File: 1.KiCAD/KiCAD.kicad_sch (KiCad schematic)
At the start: 22 parts, among them J1 Conn_02x20_Odd_Even, J10 CELL_1, J11 CELL_2, J12 CELL_3, J13 CELL_4, J2 Conn_02x20_Odd_Even, J3 TEMP, J4 TEMP, J5 BAT+, J6 BAT-, J7 LOAD+, J8 LOAD-, Q1 Charge, Q2 Discharge, Q3 Charge, Q4 Discharge, U1 MUX, U2 MUX

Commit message: BOM finished
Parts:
- added C3, C4: 100NF_50V_CER, VAMK_C_SMD:C1206, symbol VAMK_C_SMD:100NF_50V_CER
- added D1, D2: 3.3V, Diode_SMD:D_SMF, symbol Diode:BZV55B3V0
- added R3, R4, R7, R8: 10k, VAMK_R_SMD:1206, symbol VAMK_R_SMD:10k
- added R5: 1m, VAMK_R_SMD:1206, symbol VAMK_R_SMD:0R
- added R6: 160R, VAMK_R_SMD:1206, symbol VAMK_R_SMD:0R
- added U3, U4: AD8021AR, Package_SO:SOIC-8_3.9x4.9mm_P1.27mm, symbol Amplifier_Operational:AD8021AR
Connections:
- net LOAD+ is gone; now on net BAT+: J7.1 (Pin_1)
- net BAT+: now also C1.1, C4.1, R3.2, U3.8 (VS+), U4.4 (+iN), U4.8 (VS+)
- net BAT-: now also C3.2, R5.1, R6.1; no longer C1.1, Q2.1 (S), Q4.1 (S)
- net GND: now also J1.8 (Pin_8), U1.3 (GND), U2.3 (GND), R4.1, R8.1, U4.5 (VS-), U4.6 (REF)
- net PA0: now also J1.28 (Pin_28), J3.2 (Pin_2), R1.2; no longer J1.36 (Pin_36), Q2.4 (G), Q4.4 (G)
- net PA1: now also J1.30 (Pin_30), J4.2 (Pin_2), R2.2; no longer J1.34 (Pin_34), Q1.4 (G), Q3.4 (G)
- net PA4: now also J1.32 (Pin_32), D2.1 (K); no longer J1.28 (Pin_28)
- net PC0: now also J2.18 (Pin_18), Q1.4 (G), Q3.4 (G); no longer J3.2 (Pin_2), R1.2
- net PC1: now also J2.16 (Pin_16), Q2.4 (G), Q4.4 (G); no longer J2.9 (Pin_9), J4.2 (Pin_2), R2.2
- net PC2: now reaches U1.1 (A0)
- net PC2: now also J1.35 (Pin_35), U2.1 (A0)
- net PC3: now reaches U1.10 (A1)
- net PC3: now also J1.37 (Pin_37), U2.10 (A1)
- net C1+: now reaches U1.2 (S1)
- net C1+: now also J10.2 (Pin_2)
- net C3+: now reaches U1.4 (S3)
- net C3+: now also J12.2 (Pin_2)
- net PB2: now reaches U1.5 (EN)
- net PB2: now also J2.22 (Pin_22), U2.5 (EN)
- net 3.3V: now reaches U1.6 (VDD)
- net 3.3V: now also J1.16 (Pin_16), U2.6 (VDD), R7.2
- net C4+: now reaches U1.7 (S4)
- net C4+: now also J13.2 (Pin_2)
- net at U1.8 (D): now also U4.3 (RG)
- net C2+: now reaches U1.9 (S2)
- net C2+: now also J11.2 (Pin_2)
- net C1-: now reaches U2.2 (S1)
- net C1-: now also J10.1 (Pin_1)
- net C3-: now reaches U2.4 (S3)
- net C3-: now also J12.1 (Pin_1)
- net C4-: now reaches U2.7 (S4)
- net C4-: now also J13.1 (Pin_1)
- net at U2.8 (D): now also U4.2 (RG)
- net C2-: now reaches U2.9 (S2)
- net C2-: now also J11.1 (Pin_1)
- net PB0: no longer names the net of J2.14 (Pin_14)
- new net: D1.2 (A), U3.7 (Out)
- new net: Q2.1 (S), Q4.1 (S), R5.2, U3.1 (-IN)
- new net: D2.2 (A), U4.7 (Out)
- new net: R3.1, R4.2, U3.5 (VS-)
- new net: C3.1, C4.2
- new net: R7.1, R8.2, U3.6 (REF)
- new net: R6.2, U3.4 (+iN)
- new net PB1: D1.1 (K), J1.34 (Pin_34)
- no-connect marks 4 -> 71
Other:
- moved on the sheet: C1, C2, J1, J10, J11, J12, J13, J2, J3, J4, J5, J6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

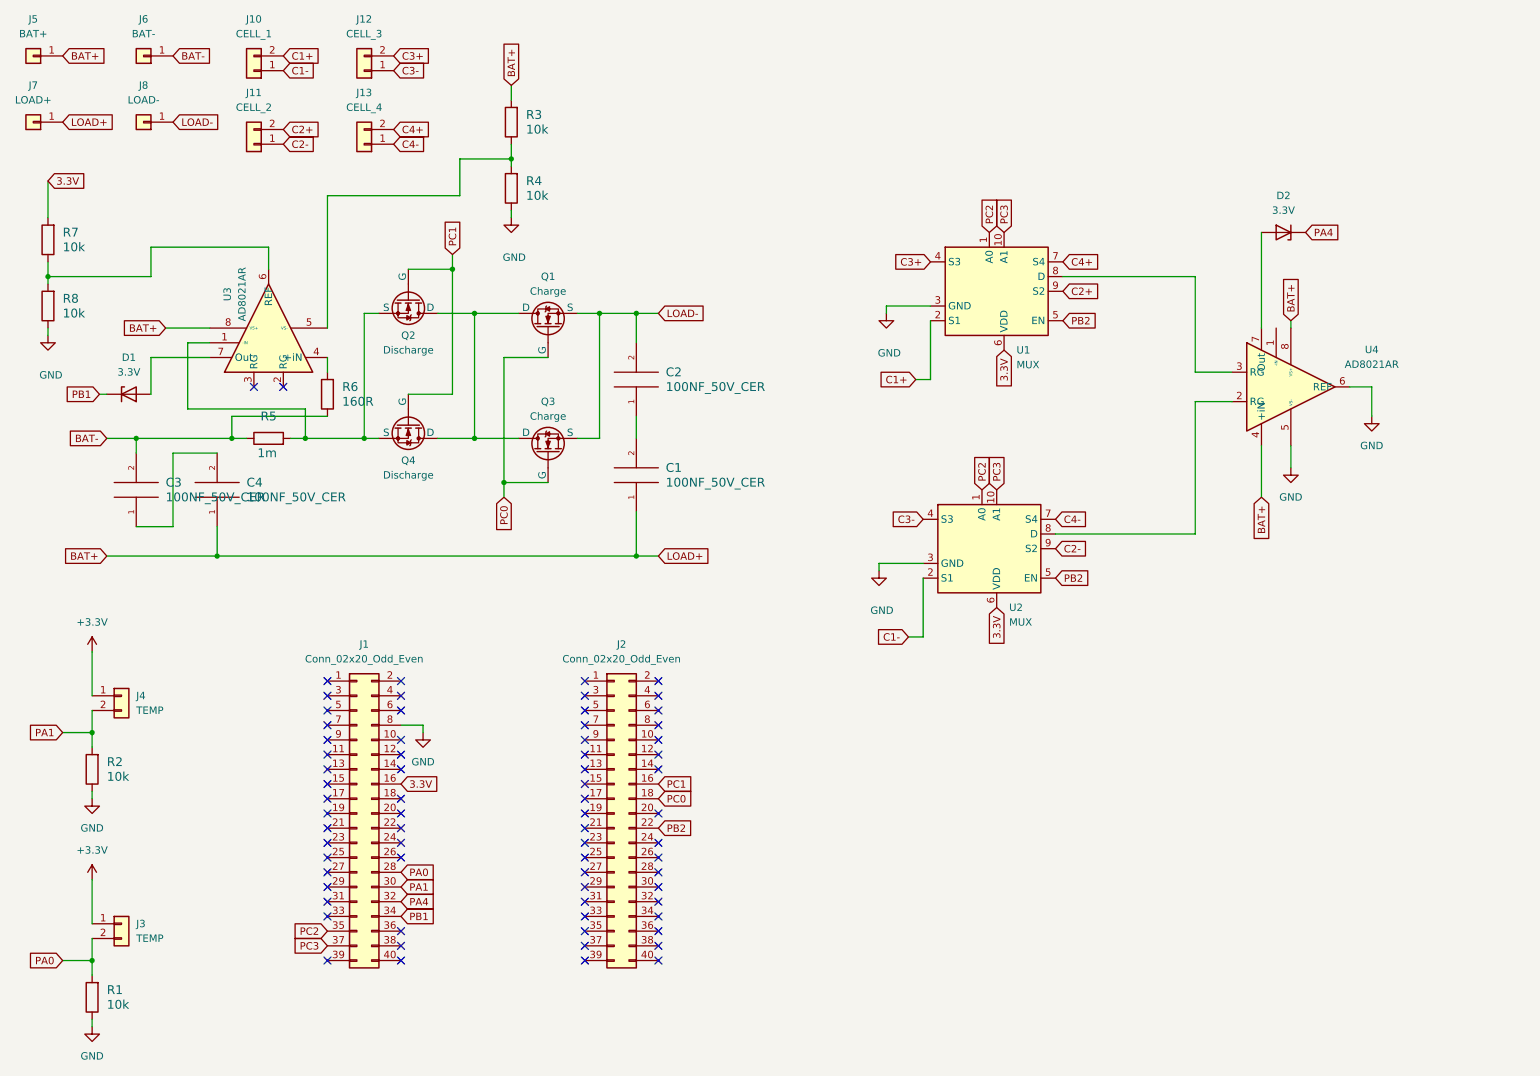
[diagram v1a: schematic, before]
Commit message: Schematic and PCB V1 done
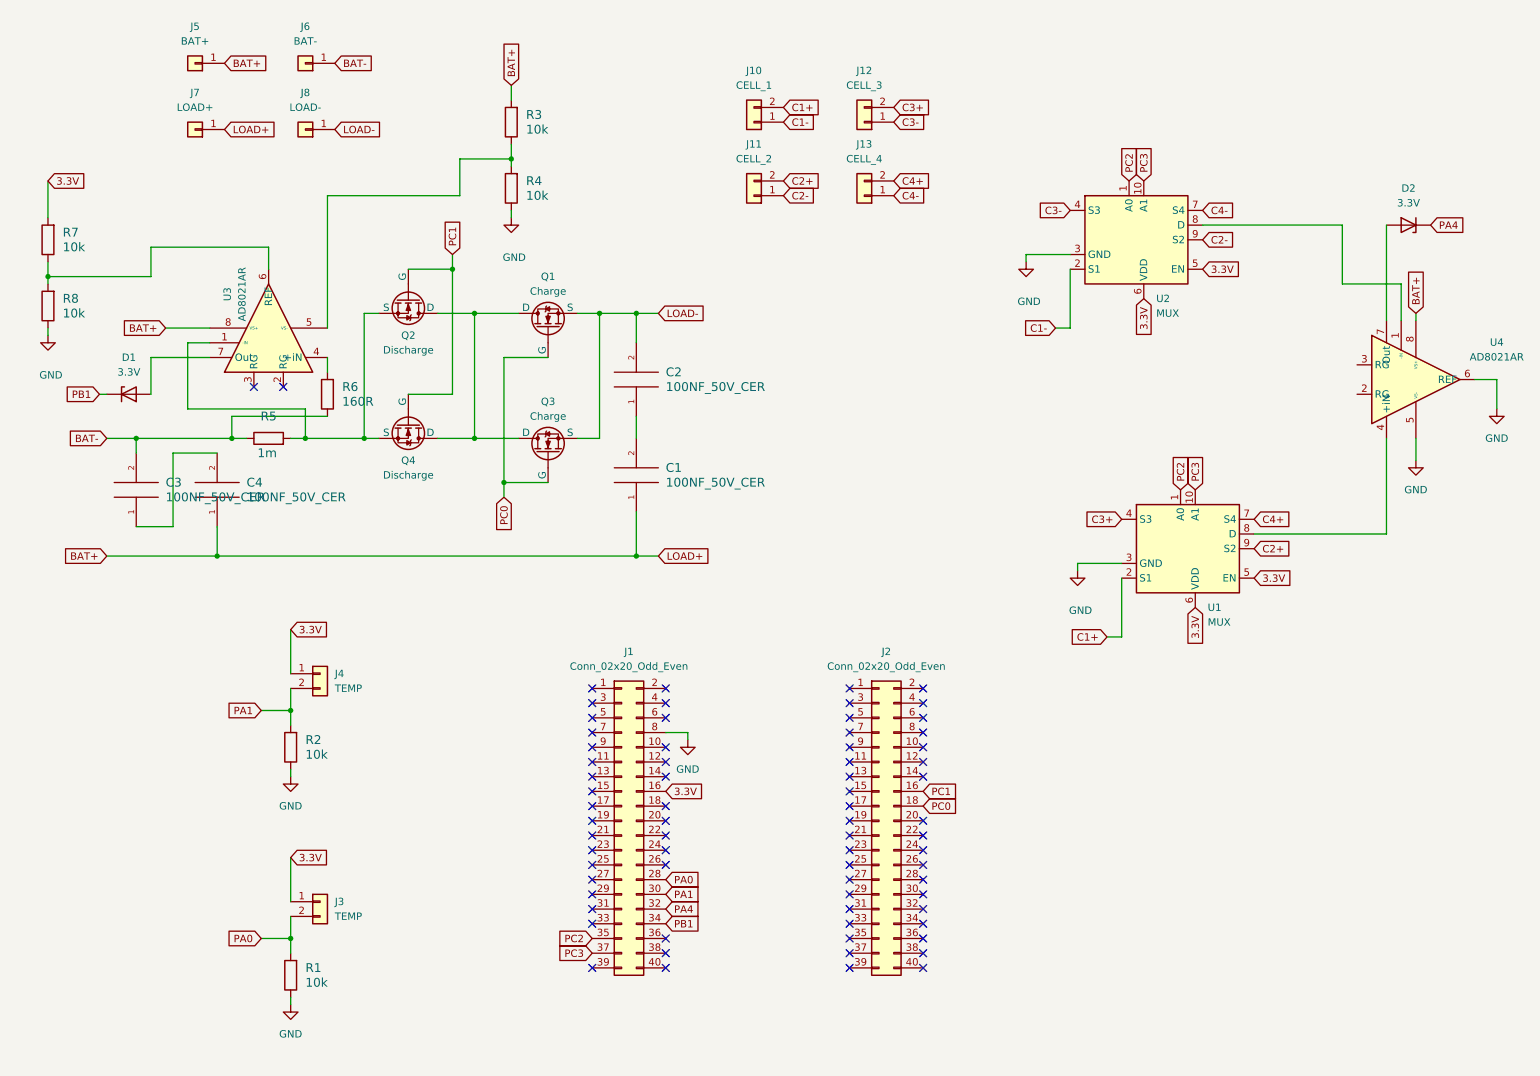
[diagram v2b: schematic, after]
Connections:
- net +3.3V is gone; now on net 3.3V: J3.1 (Pin_1), J4.1 (Pin_1)
- net 3.3V: now also U1.5 (EN), U2.5 (EN)
- net BAT+: no longer U4.4 (+iN)
- net at U1.8 (D): now also U4.4 (+iN); no longer U4.3 (RG)
- net at U2.8 (D): now also U4.1 (-IN); no longer U4.2 (RG)
- removed net PB2: J2.22 (Pin_22), U1.5 (EN), U2.5 (EN)
- no-connect marks 71 -> 72
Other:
- moved on the sheet: D2, J1, J10, J11, J12, J13, J2, J3, J4, J5, J6, J7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
